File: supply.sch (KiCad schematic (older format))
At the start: 38 parts, among them J1 MJ-3536, J2 2, J3 3, J4 1, J5 GND, J6 Conn_01x01_Female, J7 Conn_01x01_Female, J8 Conn_01x01_Female, J9 Conn_01x01_Female, SW1 TE6-1A-DC-1-PB, U1 LM5157, U2 LM386N-4/NOPB

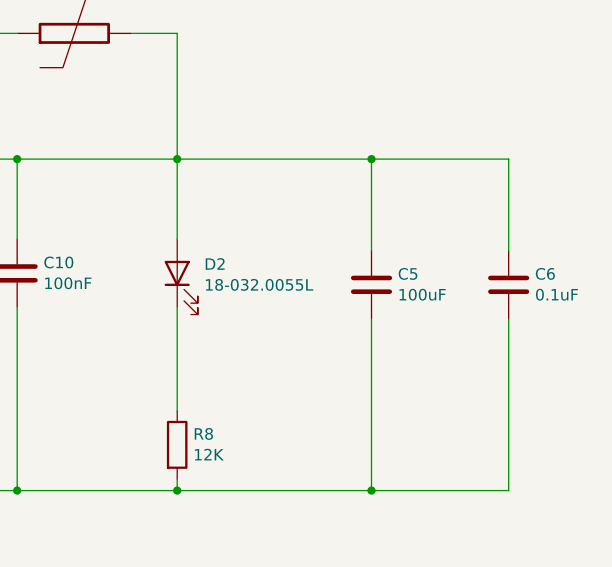
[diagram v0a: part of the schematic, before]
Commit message: Add files via upload
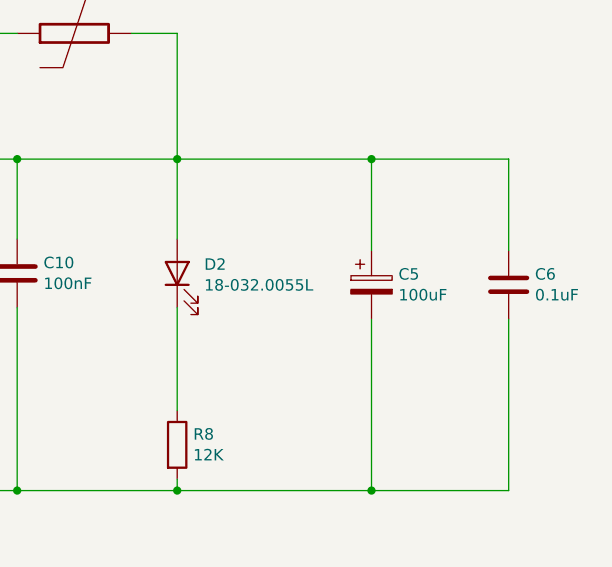
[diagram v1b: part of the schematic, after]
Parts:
- removed C5: 100uF, Capacitor_THT:C_Disc_D3.8mm_W2.6mm_P2.50mm, symbol Device:C
- added C5: 100uF, Capacitor_THT:CP_Radial_D8.0mm_P3.50mm, symbol Device:CP
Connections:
- net GND: now also C5.2
- net at C10.2, C6.2, C9.2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: now also C5.1
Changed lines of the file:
@@
 Text Label 4950 2700 0    50   ~ 0
 5
-$Comp
-L Device:C C5
-U 1 1 60D4F7C0
-P 9600 4750
-F 0 "C5" H 9485 4704 50  0000 R CNN
-F 1 "100uF" H 9485 4795 50  0000 R CNN
-F 2 "Capacitor_THT:C_Disc_D3.8mm_W2.6mm_P2.50mm" H 9638 4600 50  0001 C CNN
-F 3 "~" H 9600 4750 50  0001 C CNN
-	1    9600 4750
-	-1   0    0    1
-$EndComp
-Wire Wire Line
-	9600 4200 8750 4200
-Wire Wire Line
-	9600 4200 9600 4600
-Wire Wire Line
-	9600 4900 9600 5650
-Wire Wire Line
-	9600 5650 8750 5650
 Connection ~ 8750 5650
-$Comp
-L Device:C C6
-U 1 1 60D627B5
-P 10200 4750
-F 0 "C6" H 10085 4704 50  0000 R CNN
-F 1 "0.1uF" H 10085 4795 50  0000 R CNN
-F 2 "Capacitor_THT:C_Disc_D3.8mm_W2.6mm_P2.50mm" H 10238 4600 50  0001 C CNN
-F 3 "~" H 10200 4750 50  0001 C CNN
-	1    10200 4750
-	-1   0    0    1
-$EndComp
-Wire Wire Line
-	9600 4200 10200 4200
-Connection ~ 9600 4200
 Wire Wire Line
 	10200 4900 10200 5650
-Wire Wire Line
-	10200 5650 9600 5650
-Connection ~ 9600 5650
 Wire Wire Line
 	10200 4600 10200 4200
@@
 Wire Wire Line
 	8050 4200 8750 4200
+$Comp
+L Device:C C6
+U 1 1 60D627B5
+P 10200 4750
+F 0 "C6" H 10085 4704 50  0000 R CNN
+F 1 "0.1uF" H 10085 4795 50  0000 R CNN
+F 2 "Capacitor_THT:C_Disc_D3.8mm_W2.6mm_P2.50mm" H 10238 4600 50  0001 C CNN
+F 3 "~" H 10200 4750 50  0001 C CNN
+	1    10200 4750
+	-1   0    0    1
+$EndComp
+Wire Wire Line
+	10200 5650 9600 5650
+Wire Wire Line
+	9600 5650 8750 5650
+Connection ~ 9600 5650
+Wire Wire Line
+	9600 4900 9600 5650
+Wire Wire Line
+	9600 4200 10200 4200
+Wire Wire Line
+	9600 4200 8750 4200
+Connection ~ 9600 4200
+Wire Wire Line
+	9600 4200 9600 4600
+$Comp
+L Device:CP C5
+U 1 1 60D58BED
+P 9600 4750
+F 0 "C5" H 9718 4796 50  0000 L CNN
+F 1 "100uF" H 9718 4705 50  0000 L CNN
+F 2 "Capacitor_THT:CP_Radial_D8.0mm_P3.50mm" H 9638 4600 50  0001 C CNN
+F 3 "~" H 9600 4750 50  0001 C CNN
+	1    9600 4750
+	1    0    0    -1
+$EndComp
 $EndSCHEMATC
